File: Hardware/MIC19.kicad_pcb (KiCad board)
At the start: 2 copper layers, 160 x 70.2 mm, 100 parts, among them J101 SW_BOAT_ON, J102 ENGINE_VEL, J103 SW_PUMP1_ON, J104 SW_ENGINE_ON, J105 ENGINE_ACEL, J106 SW_PUMP2_ON, J107 SW_MPPT_ON, J108 MPPT_POT, J109 SW_PUMP3_ON, J110 SW_DMS, J111 SW_EMERGENCIA, J401 USART, J601 RJ45, J602 RJ45, Q101 BCV27, U201 MCP2551-I/SN, U202 MCP2515-xSO, U401 ATMEGA328P-PU, U501 LM7805, Y201 16MHz, Y401 16MHz

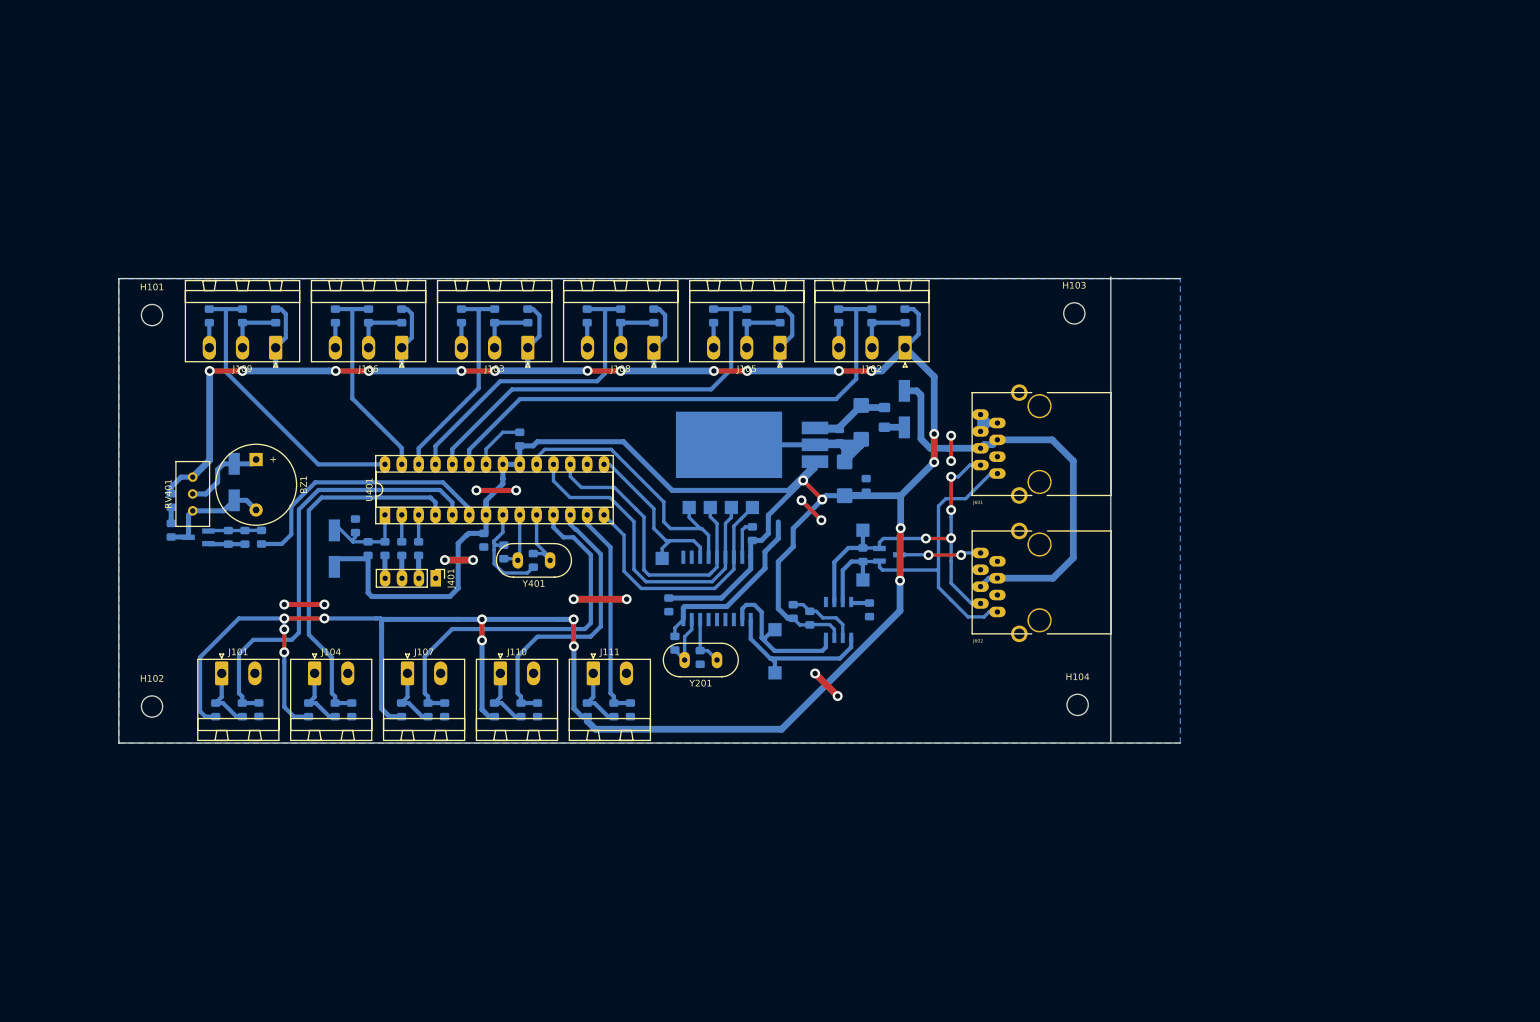
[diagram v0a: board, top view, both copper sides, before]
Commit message: Conferido e Finalizado
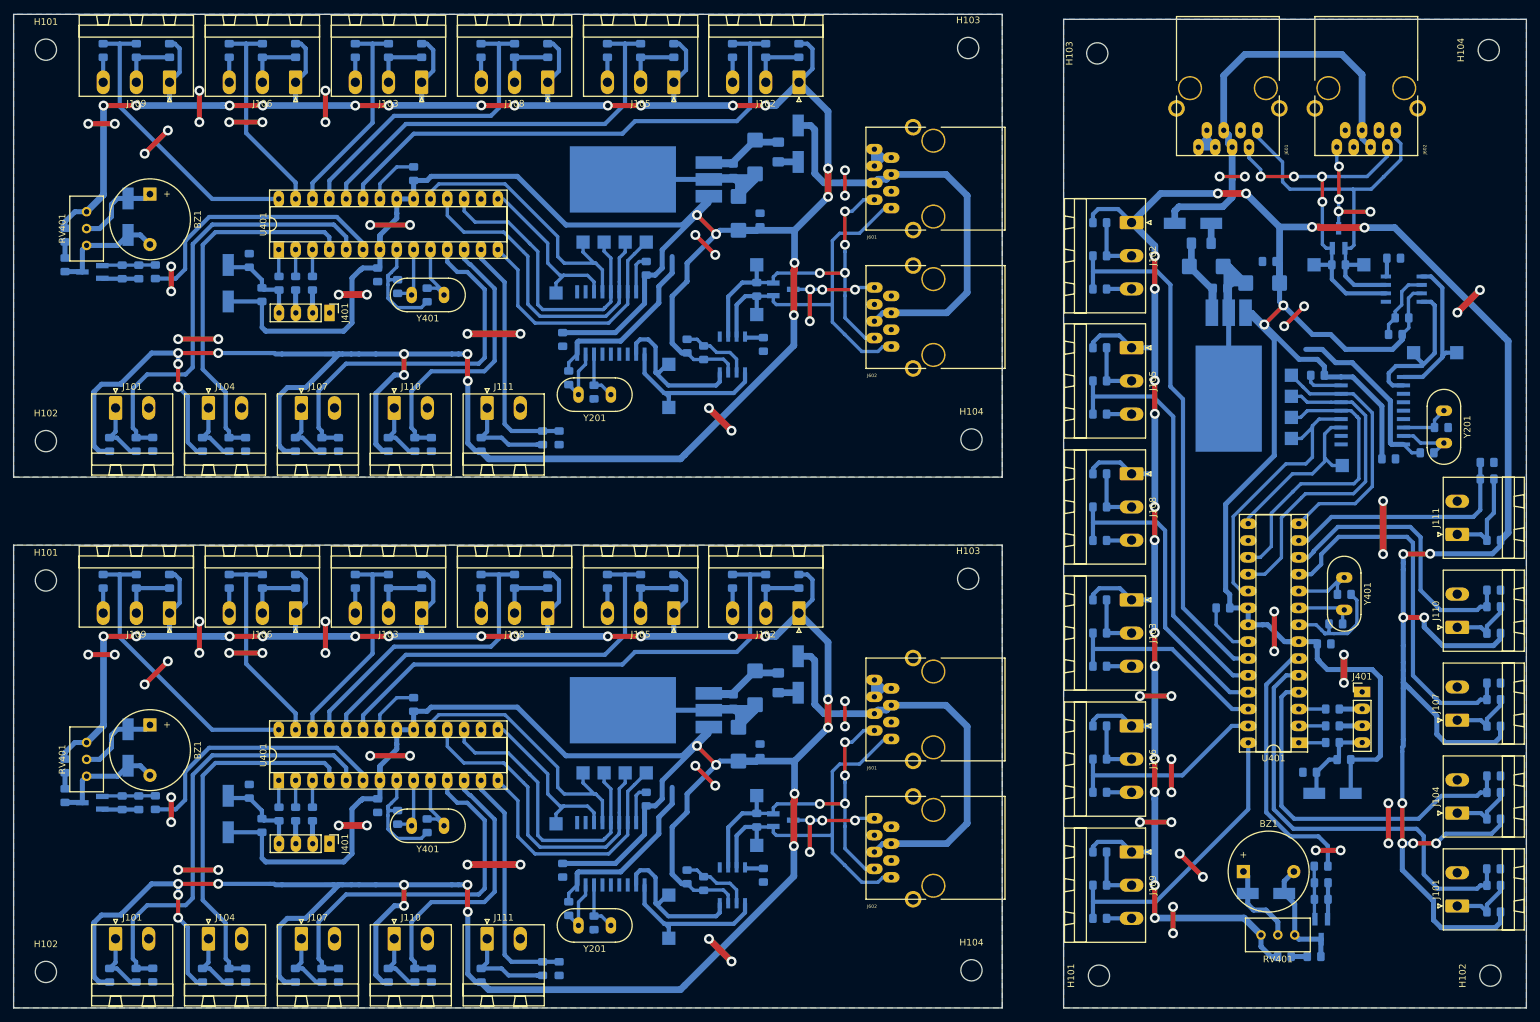
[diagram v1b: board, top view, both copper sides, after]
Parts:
- removed C405: 100nF, Capacitor_SMD:C_0805_2012Metric_Pad1.15x1.40mm_HandSolder
- added BZ1: Buzzer, Buzzer_Beeper:Buzzer_12x9.5RM7.6, F.Cu at (221.3, 158.4)
- added BZ1: Buzzer, Buzzer_Beeper:Buzzer_12x9.5RM7.6, F.Cu at (56.5, 136.3)
- added C101: 100n, Capacitor_SMD:C_0805_2012Metric_Pad1.15x1.40mm_HandSolder, B.Cu at (259.1, 158.0)
- added C101: 100n, Capacitor_SMD:C_0805_2012Metric_Pad1.15x1.40mm_HandSolder, B.Cu at (57.0, 174.1)
- added C102: 100n, Capacitor_SMD:C_0805_2012Metric_Pad1.15x1.40mm_HandSolder, B.Cu at (199.7, 70.7)
- added C102: 100n, Capacitor_SMD:C_0805_2012Metric_Pad1.15x1.40mm_HandSolder, B.Cu at (144.3, 114.7)
- added C103: 100n, Capacitor_SMD:C_0805_2012Metric_Pad1.15x1.40mm_HandSolder, B.Cu at (199.7, 127.5)
- added C103: 100n, Capacitor_SMD:C_0805_2012Metric_Pad1.15x1.40mm_HandSolder, B.Cu at (87.5, 114.7)
- added C104: 100n, Capacitor_SMD:C_0805_2012Metric_Pad1.15x1.40mm_HandSolder, B.Cu at (259.1, 144.0)
- added C104: 100n, Capacitor_SMD:C_0805_2012Metric_Pad1.15x1.40mm_HandSolder, B.Cu at (71.0, 174.1)
- added C105: 100n, Capacitor_SMD:C_0805_2012Metric_Pad1.15x1.40mm_HandSolder, B.Cu at (199.7, 89.5)
- added C105: 100n, Capacitor_SMD:C_0805_2012Metric_Pad1.15x1.40mm_HandSolder, B.Cu at (125.5, 114.7)
- added C106: 100n, Capacitor_SMD:C_0805_2012Metric_Pad1.15x1.40mm_HandSolder, B.Cu at (199.7, 146.5)
- added C106: 100n, Capacitor_SMD:C_0805_2012Metric_Pad1.15x1.40mm_HandSolder, B.Cu at (68.5, 114.7)
- added C107: 100n, Capacitor_SMD:C_0805_2012Metric_Pad1.15x1.40mm_HandSolder, B.Cu at (259.1, 130.0)
- added C107: 100n, Capacitor_SMD:C_0805_2012Metric_Pad1.15x1.40mm_HandSolder, B.Cu at (85.0, 174.1)
- added C108: 100n, Capacitor_SMD:C_0805_2012Metric_Pad1.15x1.40mm_HandSolder, B.Cu at (199.7, 108.5)
- added C108: 100n, Capacitor_SMD:C_0805_2012Metric_Pad1.15x1.40mm_HandSolder, B.Cu at (106.5, 114.7)
- added C109: 100n, Capacitor_SMD:C_0805_2012Metric_Pad1.15x1.40mm_HandSolder, B.Cu at (199.7, 165.5)
- added C109: 100n, Capacitor_SMD:C_0805_2012Metric_Pad1.15x1.40mm_HandSolder, B.Cu at (49.5, 114.7)
- added C110: 100n, Capacitor_SMD:C_0805_2012Metric_Pad1.15x1.40mm_HandSolder, B.Cu at (259.1, 116.0)
- added C110: 100n, Capacitor_SMD:C_0805_2012Metric_Pad1.15x1.40mm_HandSolder, B.Cu at (99.0, 174.1)
- added C111: 100n, Capacitor_SMD:C_0805_2012Metric_Pad1.15x1.40mm_HandSolder, B.Cu at (258.1, 96.8)
- added C111: 100n, Capacitor_SMD:C_0805_2012Metric_Pad1.15x1.40mm_HandSolder, B.Cu at (118.2, 173.1)
- added C201: 100nF, Capacitor_SMD:C_0805_2012Metric_Pad1.15x1.40mm_HandSolder, B.Cu at (243.2, 96.2)
- added C201: 100nF, Capacitor_SMD:C_0805_2012Metric_Pad1.15x1.40mm_HandSolder, B.Cu at (118.8, 158.2)
- added C202: 100nF, Capacitor_SMD:C_0805_2012Metric_Pad1.15x1.40mm_HandSolder, B.Cu at (245.2, 75.0)
- added C202: 100nF, Capacitor_SMD:C_0805_2012Metric_Pad1.15x1.40mm_HandSolder, B.Cu at (140.0, 160.2)
- added C203: 22pF, Capacitor_SMD:C_0805_2012Metric_Pad1.15x1.40mm_HandSolder, B.Cu at (251.2, 91.5)
- added C203: 22pF, Capacitor_SMD:C_0805_2012Metric_Pad1.15x1.40mm_HandSolder, B.Cu at (123.5, 166.2)
- added C204: 22pF, Capacitor_SMD:C_0805_2012Metric_Pad1.15x1.40mm_HandSolder, B.Cu at (249.0, 95.3)
- added C204: 22pF, Capacitor_SMD:C_0805_2012Metric_Pad1.15x1.40mm_HandSolder, B.Cu at (119.7, 164.0)
- added C205: 100nF, Capacitor_SMD:C_0805_2012Metric_Pad1.15x1.40mm_HandSolder, B.Cu at (244.2, 77.5)
- added C205: 100nF, Capacitor_SMD:C_0805_2012Metric_Pad1.15x1.40mm_HandSolder, B.Cu at (137.5, 159.2)
- added C401: 100nF, Capacitor_SMD:C_0805_2012Metric_Pad1.15x1.40mm_HandSolder, B.Cu at (218.3, 118.7)
- added C401: 100nF, Capacitor_SMD:C_0805_2012Metric_Pad1.15x1.40mm_HandSolder, B.Cu at (96.3, 133.3)
- added C402: 100nF, Capacitor_SMD:C_0805_2012Metric_Pad1.15x1.40mm_HandSolder, B.Cu at (233.5, 124.1)
- added C402: 100nF, Capacitor_SMD:C_0805_2012Metric_Pad1.15x1.40mm_HandSolder, B.Cu at (90.9, 148.5)
- added C403: 22pF, Capacitor_SMD:C_0805_2012Metric_Pad1.15x1.40mm_HandSolder, B.Cu at (236.5, 116.7)
- added C403: 22pF, Capacitor_SMD:C_0805_2012Metric_Pad1.15x1.40mm_HandSolder, B.Cu at (98.3, 151.5)
- added C404: 22pF, Capacitor_SMD:C_0805_2012Metric_Pad1.15x1.40mm_HandSolder, B.Cu at (235.3, 121.1)
- added C404: 22pF, Capacitor_SMD:C_0805_2012Metric_Pad1.15x1.40mm_HandSolder, B.Cu at (93.9, 150.3)
- added C406: 10nF, Capacitor_SMD:C_0805_2012Metric_Pad1.15x1.40mm_HandSolder, B.Cu at (231.3, 143.5)
- added C406: 10nF, Capacitor_SMD:C_0805_2012Metric_Pad1.15x1.40mm_HandSolder, B.Cu at (71.5, 146.3)
- added C407: 100nF, Capacitor_SMD:C_0805_2012Metric_Pad1.15x1.40mm_HandSolder, B.Cu at (233.1, 162.6)
- added C407: 100nF, Capacitor_SMD:C_0805_2012Metric_Pad1.15x1.40mm_HandSolder, B.Cu at (52.4, 148.1)
- added C501: 1uF, Capacitor_Tantalum_SMD:CP_EIA-6032-20_AVX-F_Pad2.25x2.35mm_HandSolder, B.Cu at (215.8, 67.2)
- added C501: 1uF, Capacitor_Tantalum_SMD:CP_EIA-6032-20_AVX-F_Pad2.25x2.35mm_HandSolder, B.Cu at (147.8, 130.8)
- added C502: 100nF, Capacitor_SMD:C_0805_2012Metric_Pad1.15x1.40mm_HandSolder, B.Cu at (217.8, 70.5)
- added C502: 100nF, Capacitor_SMD:C_0805_2012Metric_Pad1.15x1.40mm_HandSolder, B.Cu at (144.5, 132.8)
- added C503: 100nF, Capacitor_SMD:C_0805_2012Metric_Pad1.15x1.40mm_HandSolder, B.Cu at (225.2, 66.5)
- added C503: 100nF, Capacitor_SMD:C_0805_2012Metric_Pad1.15x1.40mm_HandSolder, B.Cu at (148.5, 140.2)
- added C504: 1uF, Capacitor_Tantalum_SMD:CP_EIA-6032-20_AVX-F_Pad2.25x2.35mm_HandSolder, B.Cu at (224.2, 69.8)
- added C504: 1uF, Capacitor_Tantalum_SMD:CP_EIA-6032-20_AVX-F_Pad2.25x2.35mm_HandSolder, B.Cu at (145.2, 139.2)
- added D201: pesd1can, Package_TO_SOT_SMD:SOT-23_Handsoldering, B.Cu at (235.7, 63.0)
- added D201: pesd1can, Package_TO_SOT_SMD:SOT-23_Handsoldering, B.Cu at (152.0, 150.7)
- added D401: LL4148, Diode_SMD:D_MiniMELF_Handsoldering, B.Cu at (234.8, 146.7)
- added D401: LL4148, Diode_SMD:D_MiniMELF_Handsoldering, B.Cu at (68.3, 149.8)
- added D402: BYD77, Diode_SMD:D_MiniMELF_Handsoldering, B.Cu at (224.8, 161.8)
- added D402: BYD77, Diode_SMD:D_MiniMELF_Handsoldering, B.Cu at (53.2, 139.8)
- added D403: LED_RED, LED_SMD:LED_0805_2012Metric_Pad1.15x1.40mm_HandSolder, B.Cu at (232.0, 171.2)
- added D403: LED_RED, LED_SMD:LED_0805_2012Metric_Pad1.15x1.40mm_HandSolder, B.Cu at (43.8, 147.0)
- added D501: LL4148, Diode_SMD:D_MiniMELF_Handsoldering, B.Cu at (213.8, 60.8)
- added D501: LL4148, Diode_SMD:D_MiniMELF_Handsoldering, B.Cu at (154.2, 128.8)
- added F501: 500mA, Fuse:Fuse_1206_3216Metric_Pad1.42x1.75mm_HandSolder, B.Cu at (215.0, 63.8)
- added F501: 500mA, Fuse:Fuse_1206_3216Metric_Pad1.42x1.75mm_HandSolder, B.Cu at (151.2, 130.0)
- added H101: MountingHole, MountingHole:MountingHole_3.2mm_M3, F.Cu at (199.6, 174.1)
- added H101: MountingHole, MountingHole:MountingHole_3.2mm_M3, F.Cu at (40.9, 114.6)
- added H102: MountingHole, MountingHole:MountingHole_3.2mm_M3, F.Cu at (258.6, 174.1)
- added H102: MountingHole, MountingHole:MountingHole_3.2mm_M3, F.Cu at (40.9, 173.6)
- added H103: MountingHole, MountingHole:MountingHole_3.2mm_M3, F.Cu at (199.3, 35.1)
- added H103: MountingHole, MountingHole:MountingHole_3.2mm_M3, F.Cu at (179.9, 114.3)
- added H104: MountingHole, MountingHole:MountingHole_3.2mm_M3, F.Cu at (258.3, 34.6)
- added H104: MountingHole, MountingHole:MountingHole_3.2mm_M3, F.Cu at (180.4, 173.3)
- added J101: SW_BOAT_ON, Connector_Phoenix_MSTB:PhoenixContact_MSTBA_2,5_2-G_1x02_P5.00mm_Horizontal, F.Cu at (253.6, 163.6)
- added J101: SW_BOAT_ON, Connector_Phoenix_MSTB:PhoenixContact_MSTBA_2,5_2-G_1x02_P5.00mm_Horizontal, F.Cu at (51.4, 168.6)
- added J102: ENGINE_VEL, Connector_Phoenix_MSTB:PhoenixContact_MSTBA_2,5_3-G_1x03_P5.00mm_Horizontal, F.Cu at (204.5, 60.6)
- added J102: ENGINE_VEL, Connector_Phoenix_MSTB:PhoenixContact_MSTBA_2,5_3-G_1x03_P5.00mm_Horizontal, F.Cu at (154.4, 119.5)
- added J103: SW_PUMP1_ON, Connector_Phoenix_MSTB:PhoenixContact_MSTBA_2,5_3-G_1x03_P5.00mm_Horizontal, F.Cu at (204.5, 117.5)
- added J103: SW_PUMP1_ON, Connector_Phoenix_MSTB:PhoenixContact_MSTBA_2,5_3-G_1x03_P5.00mm_Horizontal, F.Cu at (97.5, 119.5)
- added J104: SW_ENGINE_ON, Connector_Phoenix_MSTB:PhoenixContact_MSTBA_2,5_2-G_1x02_P5.00mm_Horizontal, F.Cu at (253.6, 149.6)
- added J104: SW_ENGINE_ON, Connector_Phoenix_MSTB:PhoenixContact_MSTBA_2,5_2-G_1x02_P5.00mm_Horizontal, F.Cu at (65.4, 168.6)
- added J105: ENGINE_ACEL, Connector_Phoenix_MSTB:PhoenixContact_MSTBA_2,5_3-G_1x03_P5.00mm_Horizontal, F.Cu at (204.5, 79.5)
- added J105: ENGINE_ACEL, Connector_Phoenix_MSTB:PhoenixContact_MSTBA_2,5_3-G_1x03_P5.00mm_Horizontal, F.Cu at (135.5, 119.5)
- added J106: SW_PUMP2_ON, Connector_Phoenix_MSTB:PhoenixContact_MSTBA_2,5_3-G_1x03_P5.00mm_Horizontal, F.Cu at (204.5, 136.5)
- added J106: SW_PUMP2_ON, Connector_Phoenix_MSTB:PhoenixContact_MSTBA_2,5_3-G_1x03_P5.00mm_Horizontal, F.Cu at (78.5, 119.5)
- added J107: SW_MPPT_ON, Connector_Phoenix_MSTB:PhoenixContact_MSTBA_2,5_2-G_1x02_P5.00mm_Horizontal, F.Cu at (253.6, 135.6)
- added J107: SW_MPPT_ON, Connector_Phoenix_MSTB:PhoenixContact_MSTBA_2,5_2-G_1x02_P5.00mm_Horizontal, F.Cu at (79.4, 168.6)
- added J108: MPPT_POT, Connector_Phoenix_MSTB:PhoenixContact_MSTBA_2,5_3-G_1x03_P5.00mm_Horizontal, F.Cu at (204.5, 98.5)
- added J108: MPPT_POT, Connector_Phoenix_MSTB:PhoenixContact_MSTBA_2,5_3-G_1x03_P5.00mm_Horizontal, F.Cu at (116.5, 119.5)
- added J109: SW_PUMP3_ON, Connector_Phoenix_MSTB:PhoenixContact_MSTBA_2,5_3-G_1x03_P5.00mm_Horizontal, F.Cu at (204.5, 155.5)
- added J109: SW_PUMP3_ON, Connector_Phoenix_MSTB:PhoenixContact_MSTBA_2,5_3-G_1x03_P5.00mm_Horizontal, F.Cu at (59.5, 119.5)
- added J110: SW_DMS, Connector_Phoenix_MSTB:PhoenixContact_MSTBA_2,5_2-G_1x02_P5.00mm_Horizontal, F.Cu at (253.6, 121.6)
- added J110: SW_DMS, Connector_Phoenix_MSTB:PhoenixContact_MSTBA_2,5_2-G_1x02_P5.00mm_Horizontal, F.Cu at (93.4, 168.6)
- added J111: SW_EMERGENCIA, Connector_Phoenix_MSTB:PhoenixContact_MSTBA_2,5_2-G_1x02_P5.00mm_Horizontal, F.Cu at (253.6, 107.6)
- added J111: SW_EMERGENCIA, Connector_Phoenix_MSTB:PhoenixContact_MSTBA_2,5_2-G_1x02_P5.00mm_Horizontal, F.Cu at (107.4, 168.6)
- added J401: USART, Connector_PinHeader_2.54mm:PinHeader_1x04_P2.54mm_Vertical, F.Cu at (239.2, 131.4)
- added J401: USART, Connector_PinHeader_2.54mm:PinHeader_1x04_P2.54mm_Vertical, F.Cu at (83.6, 154.2)
- added J601: RJ45, KicadZeniteSolarLibrary18:RJ45_YH59_01, F.Cu at (223.5, 46.7)
- added J601: RJ45, KicadZeniteSolarLibrary18:RJ45_YH59_01, F.Cu at (168.3, 138.5)
- added J602: RJ45, KicadZeniteSolarLibrary18:RJ45_YH59_01, F.Cu at (244.3, 46.7)
- added J602: RJ45, KicadZeniteSolarLibrary18:RJ45_YH59_01, F.Cu at (168.3, 159.3)
- added Q101: BCV27, Package_TO_SOT_SMD:SOT-23_Handsoldering, B.Cu at (233.1, 167.1)
- added Q101: BCV27, Package_TO_SOT_SMD:SOT-23_Handsoldering, B.Cu at (47.9, 148.1)
- added R101: 10k, Resistor_SMD:R_0805_2012Metric_Pad1.15x1.40mm_HandSolder, B.Cu at (259.1, 164.5)
- added R101: 10k, Resistor_SMD:R_0805_2012Metric_Pad1.15x1.40mm_HandSolder, B.Cu at (50.5, 174.1)
- added R102: 10k, Resistor_SMD:R_0805_2012Metric_Pad1.15x1.40mm_HandSolder, B.Cu at (199.7, 60.6)
- added R102: 10k, Resistor_SMD:R_0805_2012Metric_Pad1.15x1.40mm_HandSolder, B.Cu at (154.3, 114.7)
- added R103: 10k, Resistor_SMD:R_0805_2012Metric_Pad1.15x1.40mm_HandSolder, B.Cu at (199.7, 117.5)
- added R103: 10k, Resistor_SMD:R_0805_2012Metric_Pad1.15x1.40mm_HandSolder, B.Cu at (97.5, 114.7)
- added R104: 100R, Resistor_SMD:R_0805_2012Metric_Pad1.15x1.40mm_HandSolder, B.Cu at (259.1, 160.5)
- added R104: 100R, Resistor_SMD:R_0805_2012Metric_Pad1.15x1.40mm_HandSolder, B.Cu at (54.5, 174.1)
- added R105: 100R, Resistor_SMD:R_0805_2012Metric_Pad1.15x1.40mm_HandSolder, B.Cu at (199.7, 65.7)
- added R105: 100R, Resistor_SMD:R_0805_2012Metric_Pad1.15x1.40mm_HandSolder, B.Cu at (149.3, 114.7)
- added R106: 100R, Resistor_SMD:R_0805_2012Metric_Pad1.15x1.40mm_HandSolder, B.Cu at (199.7, 122.5)
- added R106: 100R, Resistor_SMD:R_0805_2012Metric_Pad1.15x1.40mm_HandSolder, B.Cu at (92.5, 114.7)
- added R107: 10k, Resistor_SMD:R_0805_2012Metric_Pad1.15x1.40mm_HandSolder, B.Cu at (259.1, 150.5)
- added R107: 10k, Resistor_SMD:R_0805_2012Metric_Pad1.15x1.40mm_HandSolder, B.Cu at (64.5, 174.1)
- added R108: 10k, Resistor_SMD:R_0805_2012Metric_Pad1.15x1.40mm_HandSolder, B.Cu at (199.7, 79.5)
- added R108: 10k, Resistor_SMD:R_0805_2012Metric_Pad1.15x1.40mm_HandSolder, B.Cu at (135.5, 114.7)
- added R109: 10k, Resistor_SMD:R_0805_2012Metric_Pad1.15x1.40mm_HandSolder, B.Cu at (199.7, 136.5)
- added R109: 10k, Resistor_SMD:R_0805_2012Metric_Pad1.15x1.40mm_HandSolder, B.Cu at (78.5, 114.7)
- added R110: 100R, Resistor_SMD:R_0805_2012Metric_Pad1.15x1.40mm_HandSolder, B.Cu at (259.1, 146.5)
- added R110: 100R, Resistor_SMD:R_0805_2012Metric_Pad1.15x1.40mm_HandSolder, B.Cu at (68.5, 174.1)
- added R111: 100R, Resistor_SMD:R_0805_2012Metric_Pad1.15x1.40mm_HandSolder, B.Cu at (199.7, 84.5)
- added R111: 100R, Resistor_SMD:R_0805_2012Metric_Pad1.15x1.40mm_HandSolder, B.Cu at (130.5, 114.7)
- added R112: 100R, Resistor_SMD:R_0805_2012Metric_Pad1.15x1.40mm_HandSolder, B.Cu at (199.7, 141.5)
- added R112: 100R, Resistor_SMD:R_0805_2012Metric_Pad1.15x1.40mm_HandSolder, B.Cu at (73.5, 114.7)
- added R113: 10k, Resistor_SMD:R_0805_2012Metric_Pad1.15x1.40mm_HandSolder, B.Cu at (259.1, 136.5)
- added R113: 10k, Resistor_SMD:R_0805_2012Metric_Pad1.15x1.40mm_HandSolder, B.Cu at (78.5, 174.1)
- added R114: 10k, Resistor_SMD:R_0805_2012Metric_Pad1.15x1.40mm_HandSolder, B.Cu at (199.7, 98.5)
- added R114: 10k, Resistor_SMD:R_0805_2012Metric_Pad1.15x1.40mm_HandSolder, B.Cu at (116.5, 114.7)
- added R115: 10k, Resistor_SMD:R_0805_2012Metric_Pad1.15x1.40mm_HandSolder, B.Cu at (199.7, 155.5)
- added R115: 10k, Resistor_SMD:R_0805_2012Metric_Pad1.15x1.40mm_HandSolder, B.Cu at (59.5, 114.7)
- added R116: 100R, Resistor_SMD:R_0805_2012Metric_Pad1.15x1.40mm_HandSolder, B.Cu at (259.1, 132.5)
- added R116: 100R, Resistor_SMD:R_0805_2012Metric_Pad1.15x1.40mm_HandSolder, B.Cu at (82.5, 174.1)
- added R117: 100R, Resistor_SMD:R_0805_2012Metric_Pad1.15x1.40mm_HandSolder, B.Cu at (199.7, 103.5)
- added R117: 100R, Resistor_SMD:R_0805_2012Metric_Pad1.15x1.40mm_HandSolder, B.Cu at (111.5, 114.7)
- added R118: 100R, Resistor_SMD:R_0805_2012Metric_Pad1.15x1.40mm_HandSolder, B.Cu at (199.7, 160.5)
- added R118: 100R, Resistor_SMD:R_0805_2012Metric_Pad1.15x1.40mm_HandSolder, B.Cu at (54.5, 114.7)
- added R119: 10k, Resistor_SMD:R_0805_2012Metric_Pad1.15x1.40mm_HandSolder, B.Cu at (259.1, 122.5)
- added R119: 10k, Resistor_SMD:R_0805_2012Metric_Pad1.15x1.40mm_HandSolder, B.Cu at (92.5, 174.1)
- added R120: 100R, Resistor_SMD:R_0805_2012Metric_Pad1.15x1.40mm_HandSolder, B.Cu at (259.1, 118.5)
- added R120: 100R, Resistor_SMD:R_0805_2012Metric_Pad1.15x1.40mm_HandSolder, B.Cu at (96.5, 174.1)
- added R121: 10k, Resistor_SMD:R_0805_2012Metric_Pad1.15x1.40mm_HandSolder, B.Cu at (259.1, 108.5)
- added R121: 10k, Resistor_SMD:R_0805_2012Metric_Pad1.15x1.40mm_HandSolder, B.Cu at (106.5, 174.1)
- added R122: 100R, Resistor_SMD:R_0805_2012Metric_Pad1.15x1.40mm_HandSolder, B.Cu at (258.1, 99.3)
- added R122: 100R, Resistor_SMD:R_0805_2012Metric_Pad1.15x1.40mm_HandSolder, B.Cu at (115.7, 173.1)
- added R201: 120, Resistor_SMD:R_0805_2012Metric_Pad1.15x1.40mm_HandSolder, B.Cu at (235.7, 67.0)
- added R201: 120, Resistor_SMD:R_0805_2012Metric_Pad1.15x1.40mm_HandSolder, B.Cu at (148.0, 150.7)
- added R202: 4k7, Resistor_SMD:R_0805_2012Metric_Pad1.15x1.40mm_HandSolder, B.Cu at (244.0, 66.0)
- added R202: 4k7, Resistor_SMD:R_0805_2012Metric_Pad1.15x1.40mm_HandSolder, B.Cu at (149.0, 159.0)
- added R203: 10k, Resistor_SMD:R_0805_2012Metric_Pad1.15x1.40mm_HandSolder, B.Cu at (232.5, 83.7)
- added R203: 10k, Resistor_SMD:R_0805_2012Metric_Pad1.15x1.40mm_HandSolder, B.Cu at (131.3, 147.5)
- added R401: 10k, Resistor_SMD:R_0805_2012Metric_Pad1.15x1.40mm_HandSolder, B.Cu at (236.5, 141.6)
- added R401: 10k, Resistor_SMD:R_0805_2012Metric_Pad1.15x1.40mm_HandSolder, B.Cu at (73.4, 151.5)
- added R402: 100R, Resistor_SMD:R_0805_2012Metric_Pad1.15x1.40mm_HandSolder, B.Cu at (234.8, 136.5)
- added R402: 100R, Resistor_SMD:R_0805_2012Metric_Pad1.15x1.40mm_HandSolder, B.Cu at (78.5, 149.8)
- added R403: 100R, Resistor_SMD:R_0805_2012Metric_Pad1.15x1.40mm_HandSolder, B.Cu at (234.8, 134.0)
- added R403: 100R, Resistor_SMD:R_0805_2012Metric_Pad1.15x1.40mm_HandSolder, B.Cu at (81.0, 149.8)
- added R404: 100R, Resistor_SMD:R_0805_2012Metric_Pad1.15x1.40mm_HandSolder, B.Cu at (233.1, 157.6)
- added R404: 100R, Resistor_SMD:R_0805_2012Metric_Pad1.15x1.40mm_HandSolder, B.Cu at (57.4, 148.1)
- added R405: 100R, Resistor_SMD:R_0805_2012Metric_Pad1.15x1.40mm_HandSolder, B.Cu at (233.1, 160.1)
- added R405: 100R, Resistor_SMD:R_0805_2012Metric_Pad1.15x1.40mm_HandSolder, B.Cu at (54.9, 148.1)
- added R406: 330, Resistor_SMD:R_0805_2012Metric_Pad1.15x1.40mm_HandSolder, B.Cu at (227.5, 171.2)
- added R406: 330, Resistor_SMD:R_0805_2012Metric_Pad1.15x1.40mm_HandSolder, B.Cu at (43.8, 142.5)
- added R407: 100R, Resistor_SMD:R_0805_2012Metric_Pad1.15x1.40mm_HandSolder, B.Cu at (234.8, 139.0)
- added R407: 100R, Resistor_SMD:R_0805_2012Metric_Pad1.15x1.40mm_HandSolder, B.Cu at (76.0, 149.8)
- added R407: 100R, Resistor_SMD:R_0805_2012Metric_Pad1.15x1.40mm_HandSolder, B.Cu at (76.0, 69.8)
- added RV401: 1K, Potentiometer_THT:Potentiometer_Bourns_3296W_Vertical, F.Cu at (224.0, 168.0)
- added RV401: 1K, Potentiometer_THT:Potentiometer_Bourns_3296W_Vertical, F.Cu at (47.0, 139.0)
- added TP201: SI, TestPoint:TestPoint_Pad_2.0x2.0mm, B.Cu at (228.6, 90.0)
- added TP201: SI, TestPoint:TestPoint_Pad_2.0x2.0mm, B.Cu at (125.0, 143.6)
- added TP202: SO, TestPoint:TestPoint_Pad_2.0x2.0mm, B.Cu at (228.6, 86.8)
- added TP202: SO, TestPoint:TestPoint_Pad_2.0x2.0mm, B.Cu at (128.2, 143.6)
- added TP203: TXCAN, TestPoint:TestPoint_Pad_2.0x2.0mm, B.Cu at (253.5, 80.2)
- added TP203: TXCAN, TestPoint:TestPoint_Pad_2.0x2.0mm, B.Cu at (134.8, 168.5)
- added TP204: RXCAN, TestPoint:TestPoint_Pad_2.0x2.0mm, B.Cu at (247.0, 80.2)
- added TP204: RXCAN, TestPoint:TestPoint_Pad_2.0x2.0mm, B.Cu at (134.8, 162.0)
- added TP205: SC, TestPoint:TestPoint_Pad_2.0x2.0mm, B.Cu at (228.6, 83.7)
- added TP205: SC, TestPoint:TestPoint_Pad_2.0x2.0mm, B.Cu at (131.3, 143.6)
- added TP206: SCK, TestPoint:TestPoint_Pad_2.0x2.0mm, B.Cu at (228.6, 93.2)
- added TP206: SCK, TestPoint:TestPoint_Pad_2.0x2.0mm, B.Cu at (121.8, 143.6)
- added TP207: CAN_H, TestPoint:TestPoint_Pad_2.0x2.0mm, B.Cu at (239.5, 67.0)
- added TP207: CAN_H, TestPoint:TestPoint_Pad_2.0x2.0mm, B.Cu at (148.0, 154.5)
- added TP208: CAN_L, TestPoint:TestPoint_Pad_2.0x2.0mm, B.Cu at (232.0, 67.0)
- added TP208: CAN_L, TestPoint:TestPoint_Pad_2.0x2.0mm, B.Cu at (148.0, 147.0)
- added TP209: INT, TestPoint:TestPoint_Pad_2.0x2.0mm, B.Cu at (236.2, 97.2)
- added TP209: INT, TestPoint:TestPoint_Pad_2.0x2.0mm, B.Cu at (117.8, 151.2)
- added U201: MCP2551-I/SN, Package_SO:SOIC-8_3.9x4.9mm_P1.27mm, B.Cu at (245.5, 70.7)
- added U201: MCP2551-I/SN, Package_SO:SOIC-8_3.9x4.9mm_P1.27mm, B.Cu at (144.3, 160.5)
- added U202: MCP2515-xSO, Package_SO:SOIC-18W_7.5x11.6mm_P1.27mm, B.Cu at (240.8, 89.0)
- added U202: MCP2515-xSO, Package_SO:SOIC-18W_7.5x11.6mm_P1.27mm, B.Cu at (126.0, 155.8)
- added U401: ATMEGA328P-PU, Package_DIP:DIP-28_W7.62mm_Socket, F.Cu at (229.7, 139.0)
- added U401: ATMEGA328P-PU, Package_DIP:DIP-28_W7.62mm_Socket, F.Cu at (76.0, 144.7)
- added U501: LM7805, KicadZeniteSolarLibrary18:TO-220-3_Horizontal_TabDown_SMD, B.Cu at (216.6, 75.5)
- added U501: LM7805, KicadZeniteSolarLibrary18:TO-220-3_Horizontal_TabDown_SMD, B.Cu at (139.5, 131.6)
- added Y201: 16MHz, Crystal:Crystal_HC49-U_Vertical, F.Cu at (251.6, 89.0)
- added Y201: 16MHz, Crystal:Crystal_HC49-U_Vertical, F.Cu at (126.0, 166.6)
- added Y401: 16MHz, Crystal:Crystal_HC49-U_Vertical, F.Cu at (236.5, 114.1)
- added Y401: 16MHz, Crystal:Crystal_HC49-U_Vertical, F.Cu at (100.9, 151.5)
- C406: value 100nF -> 10nF
- R402, R403: value 1k -> 100R
- moved C102 43.1 mm to (144.3, 34.7)
- moved C103 43.1 mm to (87.5, 34.7)
- moved C104 43.1 mm to (71.0, 94.1)
- moved C105 43.1 mm to (125.5, 34.7)
- moved C106 43.1 mm to (68.5, 34.7)
- moved C107 43.1 mm to (85.0, 94.1)
- moved C108 43.1 mm to (106.5, 34.7)
- moved C109 43.1 mm to (49.5, 34.7)
- moved C110 43.1 mm to (99.0, 94.1)
- moved C201 43.1 mm to (118.8, 78.2)
- moved C202 43.1 mm to (140.0, 80.2)
- moved C203 43.1 mm to (123.5, 86.2)
- moved C204 43.1 mm to (119.7, 84.0)
- moved C205 43.1 mm to (137.5, 79.2)
- moved C401 43.1 mm to (96.3, 53.3)
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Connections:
- J401 pad 4: Net-(C405-Pad2) -> /MCU/RESET
- U401 pad 1: /MCU/RESET -> Net-(R407-Pad1)
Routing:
- net (no net): track 0.00 -> 4250.7 mm, vias 0 -> 120
- net GND: track 190.2 -> 222.2 mm, vias 16 -> 30
- net +5V: track 623.3 -> 632.3 mm
- net Net-(J111-Pad1): track 9.70 -> 15.4 mm
- net /Conectores/SW_EMERGENCIA: track 32.5 -> 36.4 mm
- net Net-(R407-Pad1): track 0.00 -> 3.79 mm
- net Net-(C405-Pad2): track 3.46 -> 0.00 mm
- net /MCU/RESET: track 14.2 -> 13.4 mm
- added copper zone on B.Cu, net (none)
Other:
- board size 160 x 70.2 mm -> 228 x 149.8 mm
